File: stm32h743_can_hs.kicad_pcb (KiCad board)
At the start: 4 copper layers, 99.1 x 53.3 mm, 102 parts, among them J1 Conn_02x38_Counter_Clockwise, J2 Conn_02x38_Counter_Clockwise, J3 USB_C_Receptacle_USB2.0_16P, J4 USB_C_Receptacle_USB2.0_16P, J5 DE9_Pins_MH, J6 Conn_01x05_Pin, J7 Conn_ARM_JTAG_SWD_10, Q1 BSS138, Q2 BSS138, Q3 BSS138, SW1 SW_Push, SW2 SW_Push, U1 STM32H743IITx, U2 ST1S40IDR, U3 TPS2121RUX, U4 USB3300-EZK, U5 MCP2562-E-SN, U6 S25FL128LAGMFI013, Y1 SG-210STF, Y2 8MHz, Y3 Crystal

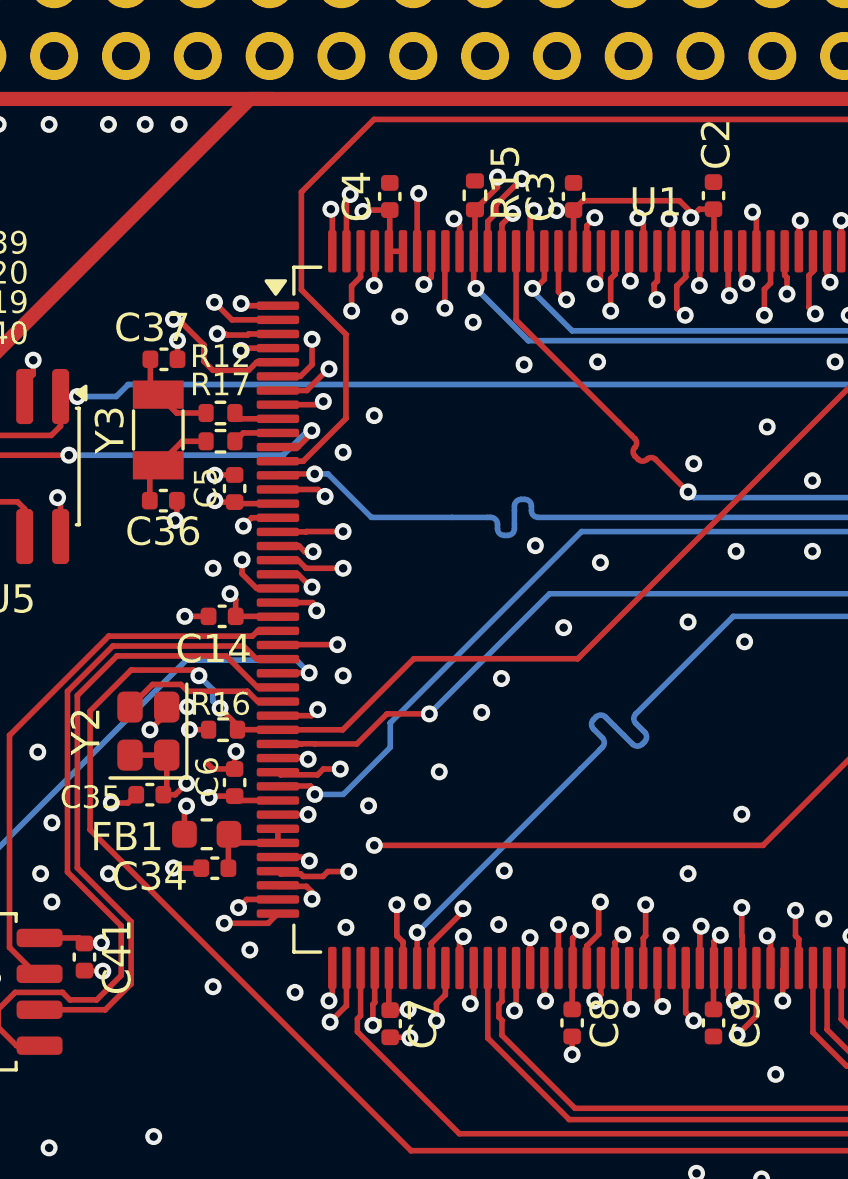
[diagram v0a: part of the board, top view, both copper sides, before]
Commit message: cleanup
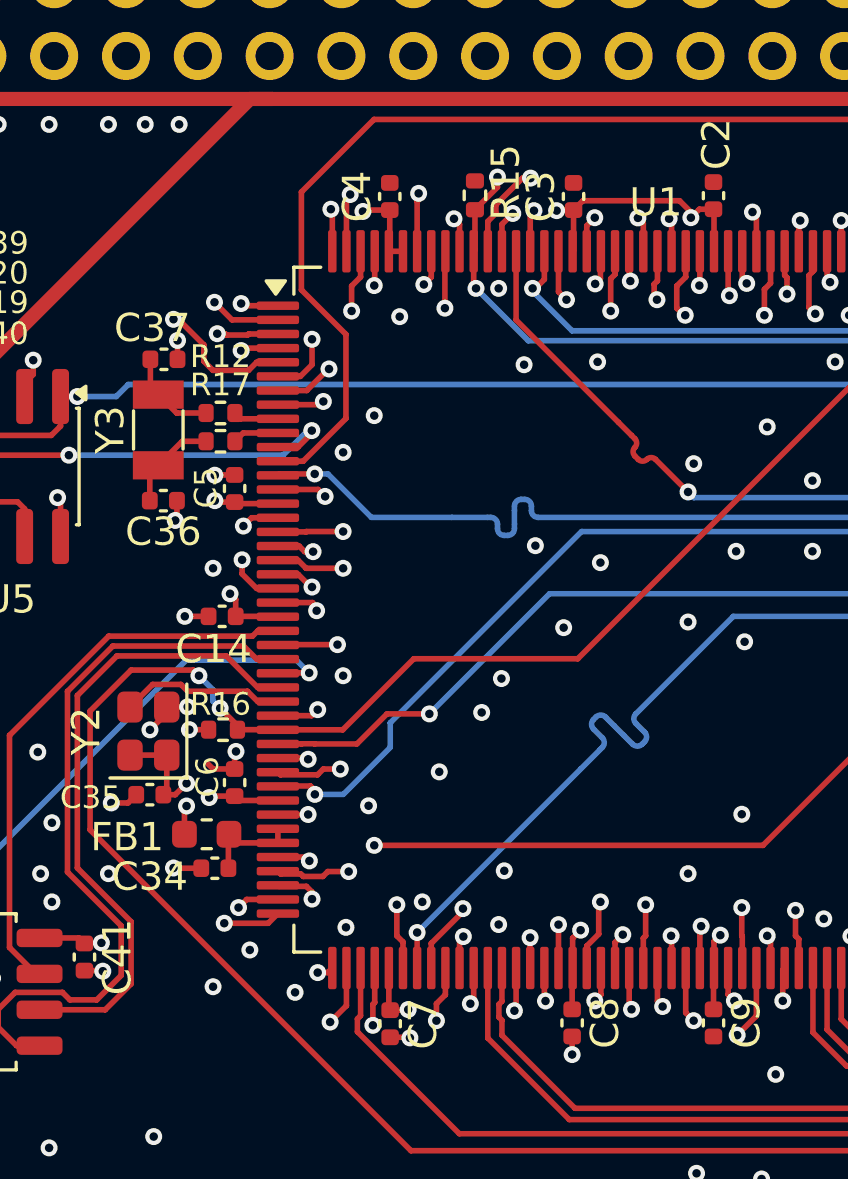
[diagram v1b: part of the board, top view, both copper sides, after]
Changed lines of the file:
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@@
 	)
 	(via
-		(at 130.7 87.5)
+		(at 131.6 86.3)
 		(size 0.6)
 		(drill 0.3)
@@
 	)
 	(segment
-		(start 125.717188 111.382812)
-		(end 125.6 111.5)
+		(start 125.2 110.5)
+		(end 125.555314 110.5)
 		(width 0.2)
 		(layer "F.Cu")
@@
 	)
 	(segment
-		(start 125.717188 110.338126)
-		(end 125.717188 111.382812)
+		(start 125.555314 110.5)
+		(end 125.717188 110.338126)
 		(width 0.2)
 		(layer "F.Cu")
@@
 	)
 	(via
-		(at 125.6 111.5)
+		(at 125.2 110.5)
 		(size 0.6)
 		(drill 0.3)
@@
 	)
 	(segment
-		(start 125.6 111.5)
-		(end 124.95 112.15)
+		(start 110.35 112.15)
+		(end 101.9 120.6)
+		(width 0.2)
+		(layer "In2.Cu")
+		(net "/PH4")
+	)
+	(segment
+		(start 125.2 110.5)
+		(end 125.2 111.9)
 		(width 0.2)
 		(layer "In2.Cu")
@@
 	)
 	(segment
-		(start 110.35 112.15)
-		(end 101.9 120.6)
+		(start 124.95 112.15)
+		(end 110.35 112.15)
 		(width 0.2)
 		(layer "In2.Cu")
@@
 	)
 	(segment
-		(start 101.9 120.6)
-		(end 101.9 122.52)
+		(start 125.2 111.9)
+		(end 124.95 112.15)
 		(width 0.2)
 		(layer "In2.Cu")
@@
 	)
 	(segment
-		(start 124.95 112.15)
-		(end 110.35 112.15)
+		(start 101.9 120.6)
+		(end 101.9 122.52)
 		(width 0.2)
 		(layer "In2.Cu")
@@
 	)
 	(segment
-		(start 131.503572 83.644956)
-		(end 131.217188 83.93134)
+		(start 131.503572 83.340792)
+		(end 131.503572 83.644956)
 		(width 0.2)
 		(layer "F.Cu")
@@
 	)
 	(segment
-		(start 131.503572 83.340792)
-		(end 131.503572 83.644956)
+		(start 132.727209 82.4)
+		(end 132.444364 82.4)
+		(width 0.2)
+		(layer "F.Cu")
+		(net "/PB7")
+	)
+	(segment
+		(start 132.444364 82.4)
+		(end 131.503572 83.340792)
 		(width 0.2)
 		(layer "F.Cu")
@@
 	)
 	(segment
-		(start 132.422182 82.422182)
-		(end 131.503572 83.340792)
+		(start 131.503572 83.644956)
+		(end 131.217188 83.93134)
 		(width 0.2)
 		(layer "F.Cu")
@@
 	)
 	(via
-		(at 132.422182 82.422182)
+		(at 132.727209 82.4)
 		(size 0.6)
 		(drill 0.3)
@@
 	)
 	(segment
-		(start 132.6 82.6)
-		(end 132.810052 82.6)
-		(width 0.2)
-		(layer "In1.Cu")
-		(net "/PB7")
-	)
-	(segment
 		(start 152.75 79.35)
 		(end 152.75 76.77)
@@
 	)
 	(segment
-		(start 132.422182 82.422182)
-		(end 132.6 82.6)
+		(start 133.010052 82.4)
+		(end 133.110052 82.3)
 		(width 0.2)
 		(layer "In1.Cu")
@@
 	)
 	(segment
-		(start 132.810052 82.6)
-		(end 133.110052 82.3)
+		(start 132.727209 82.4)
+		(end 133.010052 82.4)
 		(width 0.2)
 		(layer "In1.Cu")
@@
 	)
 	(segment
-		(start 152.75 76.77)
-		(end 153.98 75.54)
+		(start 149.8 82.3)
+		(end 152.75 79.35)
 		(width 0.2)
 		(layer "In1.Cu")
@@
 	)
 	(segment
-		(start 149.8 82.3)
-		(end 152.75 79.35)
+		(start 152.75 76.77)
+		(end 153.98 75.54)
 		(width 0.2)
 		(layer "In1.Cu")
